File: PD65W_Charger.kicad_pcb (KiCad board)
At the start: 2 copper layers, 84.6 x 64.4 mm, 28 parts, among them J1 Barrel_Jack_MountingPin, J2 Output_V-from-PD65, J3 FAN, Q1 2N2222, U1 PD65W_module, U2 OLED_0.91-I2C, U3 MOUDLE-SEEEDUINO-XIAO, U4 AP63205WU, U5 INA226

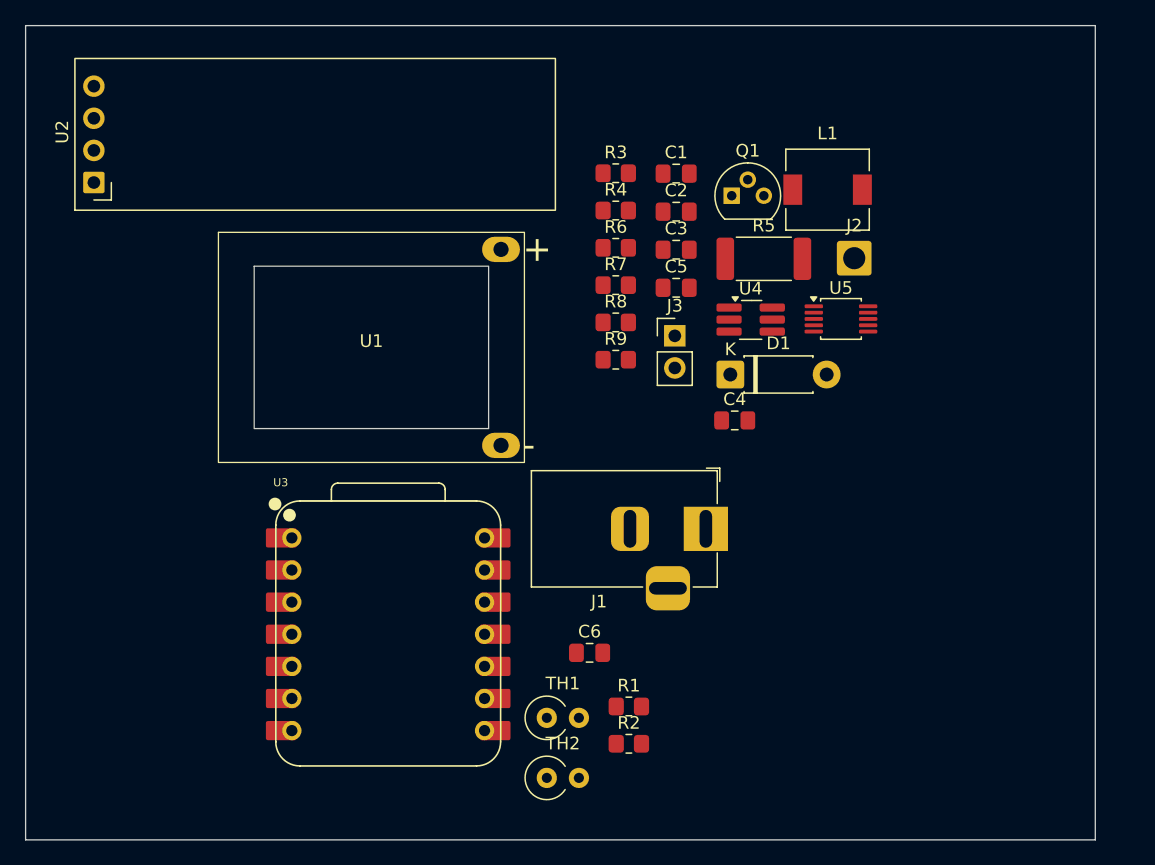
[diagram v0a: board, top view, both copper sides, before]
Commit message: upload
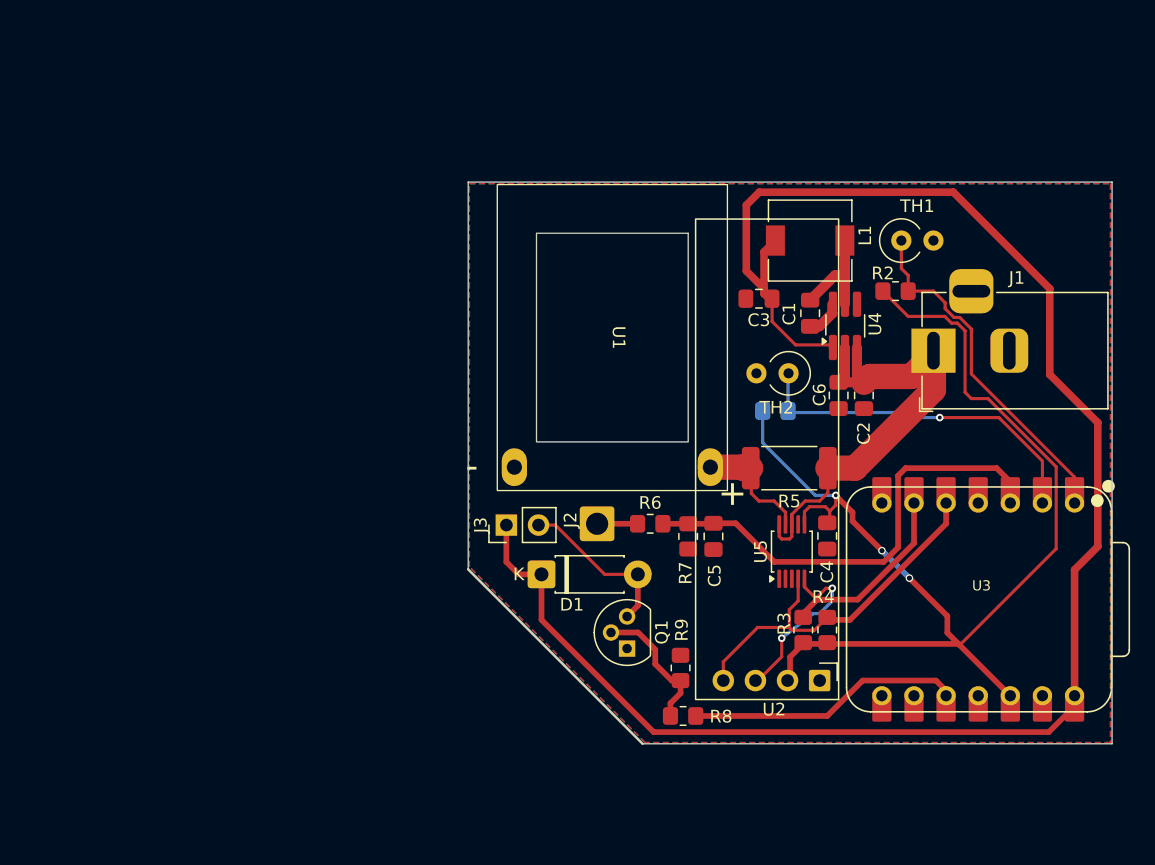
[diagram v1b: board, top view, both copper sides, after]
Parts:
- R1: moved to B.Cu
- moved U2 69.6 mm to (168.0, 110.8), turned to 180 degrees
- moved TH1 47.0 mm to (174.5, 76.0)
- moved U3 46.7 mm to (180.5, 104.4), turned to -90 degrees
- moved R2 41.5 mm to (174.0, 80.0)
- moved R3 39.0 mm to (166.7, 106.8), turned to -90 degrees
- moved TH2 37.3 mm to (165.5, 86.5), turned to 180 degrees
- moved R4 37.2 mm to (168.6, 106.8), turned to -90 degrees
- moved Q1 36.8 mm to (152.8, 108.3), turned to 90 degrees
- moved R8 31.6 mm to (157.2, 113.6), turned to 180 degrees
- moved J2 29.2 mm to (150.4, 98.4)
- moved C6 28.3 mm to (169.5, 88.2), turned to 90 degrees
- moved R1 26.1 mm to (164.5, 89.5)
- moved R9 24.9 mm to (157.0, 109.8), turned to -90 degrees
- moved J1 22.9 mm to (177.0, 84.7), turned to 180 degrees
- moved R6 22.0 mm to (154.6, 98.4)
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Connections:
- R1 pad 2: /A0 -> /A1
- R2 pad 2: /A1 -> /A0
- R8 pad 1: /D3 -> /D10
- U3 pad 10: unconnected-(U3-PA5_A9_D9_MISO-Pad10)_1 -> /D10
- U3 pad 4: /D3 -> unconnected-(U3-PA11_A3_D3-Pad4)_1
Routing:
- net +5V: track 0.00 -> 138.7 mm
- net +3V3: track 0.00 -> 93.0 mm, vias 0 -> 3
- net +24V: track 0.00 -> 38.1 mm
- net /A2: track 0.00 -> 36.4 mm
- net /SDA: track 0.00 -> 29.8 mm
- net /SCL: track 0.00 -> 28.7 mm, vias 0 -> 2
- net /A0: track 0.00 -> 27.9 mm
- net /A1: track 0.00 -> 27.1 mm, vias 0 -> 1
- net /D10: track 0.00 -> 21.7 mm
- net Net-(D1-A): track 0.00 -> 13.2 mm
- net Net-(Q1-B): track 0.00 -> 10.9 mm
- net Net-(U1-IN+): track 0.00 -> 9.87 mm
- net Net-(U4-SW): track 0.00 -> 8.60 mm
- net Net-(J2-Pin_1): track 0.00 -> 3.20 mm
- net Net-(U4-BST): track 0.00 -> 2.90 mm
- added copper zone on B.Cu, net GND
- added copper zone on F.Cu, net GND
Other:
- board size 84.6 x 64.4 mm -> 50.9 x 44.4 mm
